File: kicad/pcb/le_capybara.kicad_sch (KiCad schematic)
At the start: 24 parts, among them J1 USB_C sink board 1.3mm, J2 OLED I2C, U2 STM32F072CBT6, U3 PRTR5V0U2X

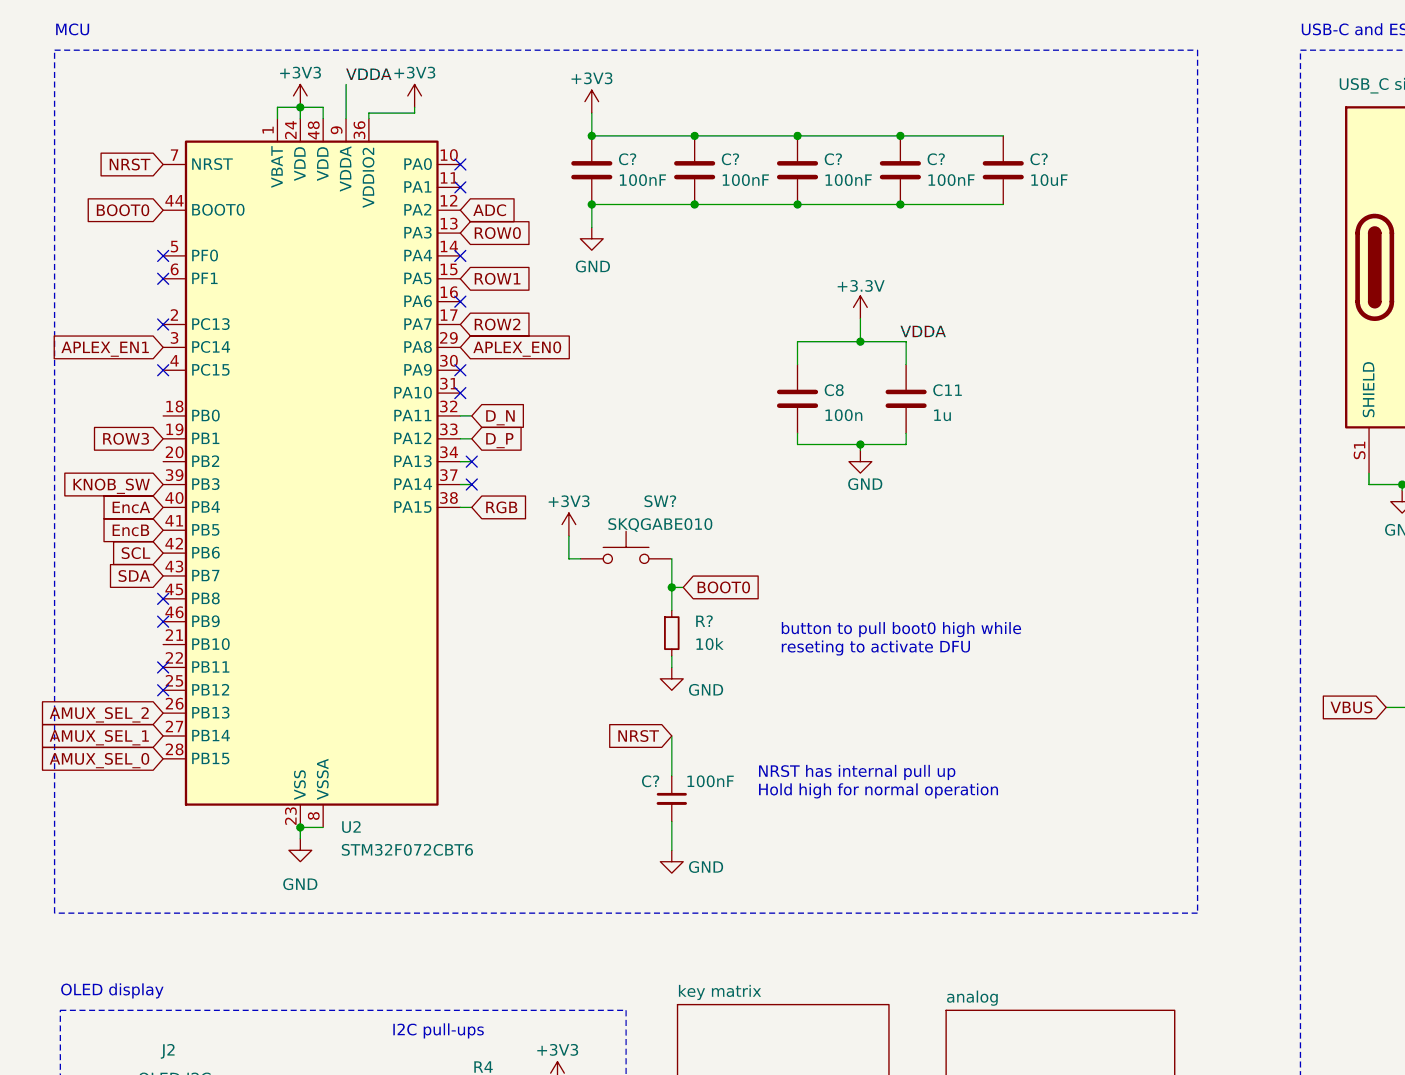
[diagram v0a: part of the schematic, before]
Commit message: getting ready for prototype
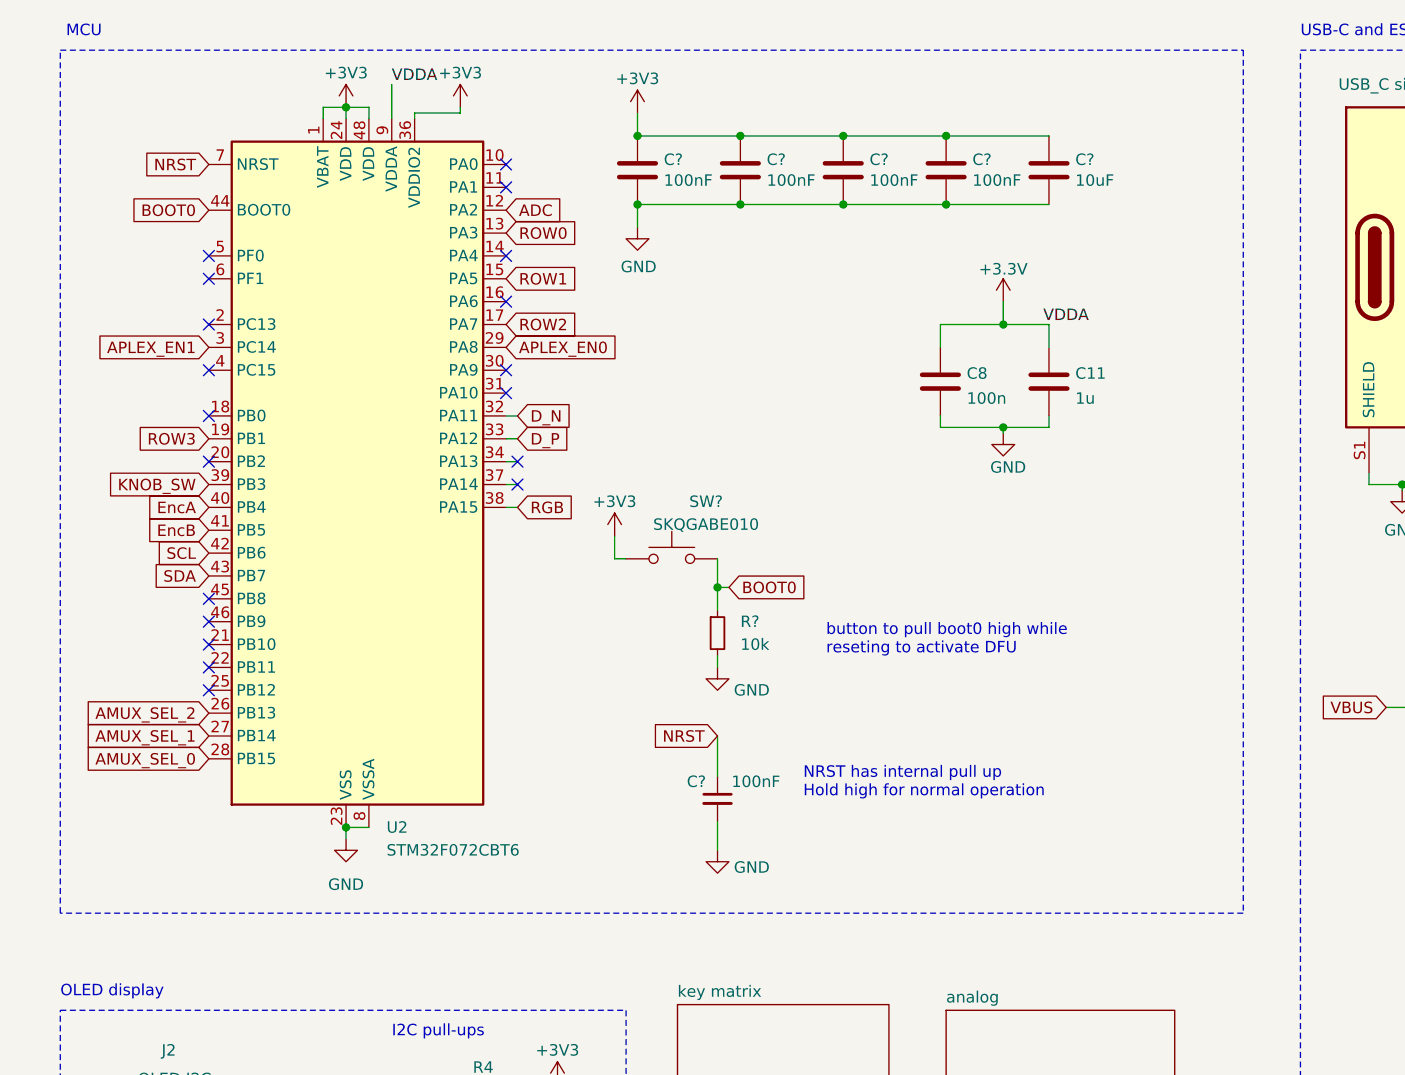
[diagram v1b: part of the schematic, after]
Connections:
- no-connect marks 18 -> 21
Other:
- moved on the sheet: C11, C8, C?, R?, SW?, U2
